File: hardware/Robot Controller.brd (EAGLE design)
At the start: 51.7 x 73 mm, 18 parts, among them U1 ATMEGA328P_PDIP

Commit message: update connections to match todays progress
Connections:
- net M1DR': now also U1.4; no longer U1.12
- net M1PW': now also U1.12; no longer U1.11
- net M2DR': now also U1.5; no longer U1.13
- net M2PW': no longer U1.5
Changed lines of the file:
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@@
 <contactref element="R1" pad="2"/>
 <contactref element="L293D" pad="1"/>
-<contactref element="U1" pad="11"/>
-<wire x1="66.04" y1="62.735" x2="62.865" y2="50.165" width="0" layer="19" extent="1-1"/>
-<wire x1="74.93" y1="38.1" x2="66.04" y2="62.735" width="0" layer="19" extent="1-1"/>
+<contactref element="U1" pad="12"/>
+<wire x1="62.865" y1="50.165" x2="66.04" y2="62.735" width="0" layer="19" extent="1-1"/>
+<wire x1="77.47" y1="38.1" x2="62.865" y2="50.165" width="0" layer="19" extent="1-1"/>
 </signal>
 <signal name="M2PW'">
 <contactref element="R3" pad="2"/>
 <contactref element="L293D" pad="9"/>
-<contactref element="U1" pad="5"/>
-<wire x1="59.69" y1="38.1" x2="69.215" y2="65.535" width="0" layer="19" extent="1-1"/>
-<wire x1="80.645" y1="57.785" x2="69.215" y2="65.535" width="0" layer="19" extent="1-1"/>
+<wire x1="69.215" y1="65.535" x2="80.645" y2="57.785" width="0" layer="19" extent="1-1"/>
 </signal>
 <signal name="M1DR'">
 <contactref element="SN74AHCU04N" pad="13"/>
 <contactref element="L293D" pad="7"/>
-<contactref element="U1" pad="12"/>
-<wire x1="78.105" y1="50.165" x2="58.42" y2="62.23" width="0" layer="19" extent="1-1"/>
-<wire x1="77.47" y1="38.1" x2="78.105" y2="50.165" width="0" layer="19" extent="1-1"/>
+<contactref element="U1" pad="4"/>
+<wire x1="58.42" y1="62.23" x2="78.105" y2="50.165" width="0" layer="19" extent="1-1"/>
+<wire x1="57.15" y1="38.1" x2="58.42" y2="62.23" width="0" layer="19" extent="1-1"/>
 </signal>
 <signal name="M2DR'">
 <contactref element="L293D" pad="10"/>
 <contactref element="SN74AHCU04N" pad="11"/>
-<contactref element="U1" pad="13"/>
+<contactref element="U1" pad="5"/>
 <wire x1="58.42" y1="57.15" x2="78.105" y2="57.785" width="0" layer="19" extent="1-1"/>
-<wire x1="80.01" y1="38.1" x2="58.42" y2="57.15" width="0" layer="19" extent="1-1"/>
+<wire x1="59.69" y1="38.1" x2="58.42" y2="57.15" width="0" layer="19" extent="1-1"/>
 </signal>
 <signal name="DEBUG'">

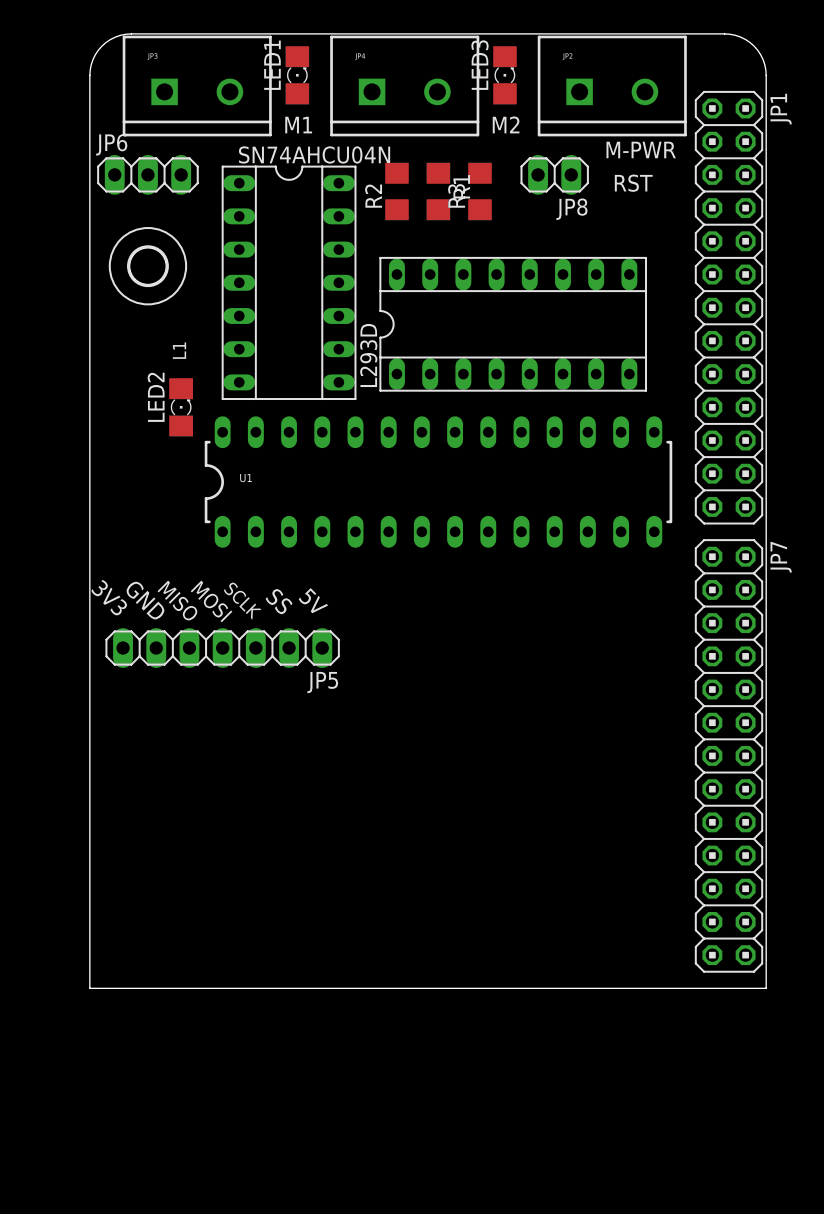
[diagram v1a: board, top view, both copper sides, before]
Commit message: WIP hardware
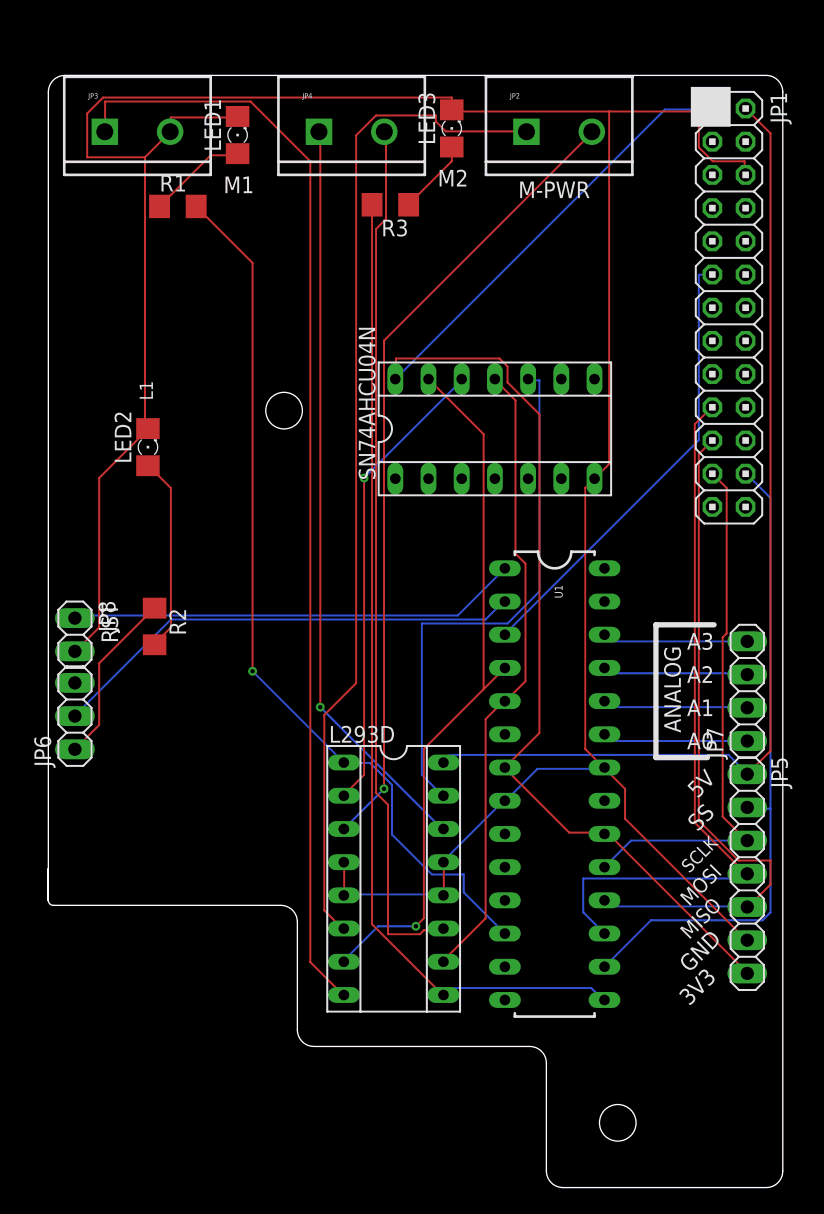
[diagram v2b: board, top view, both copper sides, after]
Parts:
- removed H1: MOUNT-HOLE2.8, holes:2,8
- JP7: device pinhead:2X13 -> pinhead:1X04
- moved JP8 50.8 mm to (38.2, 30.2), turned to 270 degrees
- moved JP5 43.7 mm to (89.7, 11.9), turned to 270 degrees
- moved L293D 43.4 mm to (62.6, 11.6), turned to 270 degrees
- moved JP6 41.8 mm to (38.2, 24.0), turned to 90 degrees
- moved R2 38.1 mm to (44.3, 30.9), turned to 270 degrees
- moved U1 24.8 mm to (74.9, 18.8), turned to 270 degrees
- moved R1 20.0 mm to (46.1, 63.0), turned to 0 degrees
- moved SN74AHCU04N 19.3 mm to (70.4, 46.0), turned to 0 degrees
- moved R3 6.93 mm to (62.4, 63.1), turned to 180 degrees
- moved LED1 6.47 mm to (50.7, 68.5)
- moved LED3 5.75 mm to (67.1, 69.0)
- moved JP3 5.49 mm to (40.5, 68.7)
- moved JP7 5.15 mm to (89.7, 25.9), turned to 90 degrees
- moved JP4 5.08 mm to (56.9, 68.7)
- moved JP2 5.08 mm to (72.8, 68.7)
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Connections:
- net DEBUG' renamed DEBUG
- removed net M2PW': L293D.9, R3.2
- new net ADC0: JP7.1, U1.23
- new net ADC1: JP7.2, U1.24
- new net ADC2: JP7.3, U1.25
- new net ADC3: JP7.4, U1.26
- new net M2PW: L293D.9, R3.2, U1.15
- net 3.3V: now also U1.20
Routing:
- net GND: track 0.00 -> 211.2 mm
- net 3.3V: track 0.00 -> 101.1 mm
- net N$10: track 0.00 -> 84.8 mm
- net N$9: track 0.00 -> 76.8 mm
- net 5V: track 0.00 -> 76.6 mm
- net M2PW: track 0.00 -> 75.7 mm
- net M1PW': track 0.00 -> 68.0 mm, vias 0 -> 1
- net N$19: track 0.00 -> 66.6 mm
- net N$8: track 0.00 -> 61.2 mm, vias 0 -> 1
- net N$18: track 0.00 -> 57.3 mm, vias 0 -> 1
- net MOSI': track 0.00 -> 55.6 mm
- net M1DR': track 0.00 -> 54.7 mm, vias 0 -> 1
- net MISO': track 0.00 -> 51.7 mm
- net SS': track 0.00 -> 50.6 mm
- net M2DR': track 0.00 -> 48.2 mm
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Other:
- board size 51.7 x 73 mm -> 56.2 x 85.1 mm
- board text added: "A0"
- board text added: "A1"
- board text added: "A2"
- board text added: "A3"
- board text added: "ANALOG"
- board text removed: ">"
